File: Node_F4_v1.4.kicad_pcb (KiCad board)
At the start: 2 copper layers, 95 x 58.5 mm, 84 parts, among them J1 Screw_Terminal_01x09, J6 Conn_01x16_Female, J7 Conn_01x08_Male, J8 STLINK, Q1 P_Mosfet, SW1 SW_Push, U10 Ai-Thinker-Ra-02, U2 PCF8574A, U3 AMS1117-3.3, U4 DS3231M, U5 MAX485E, U6 STM32F411CEUx, U7 Trans_MOSFET, U8 Trans_MOSFET, U9 W25Q128JVS, Y1 25MHz

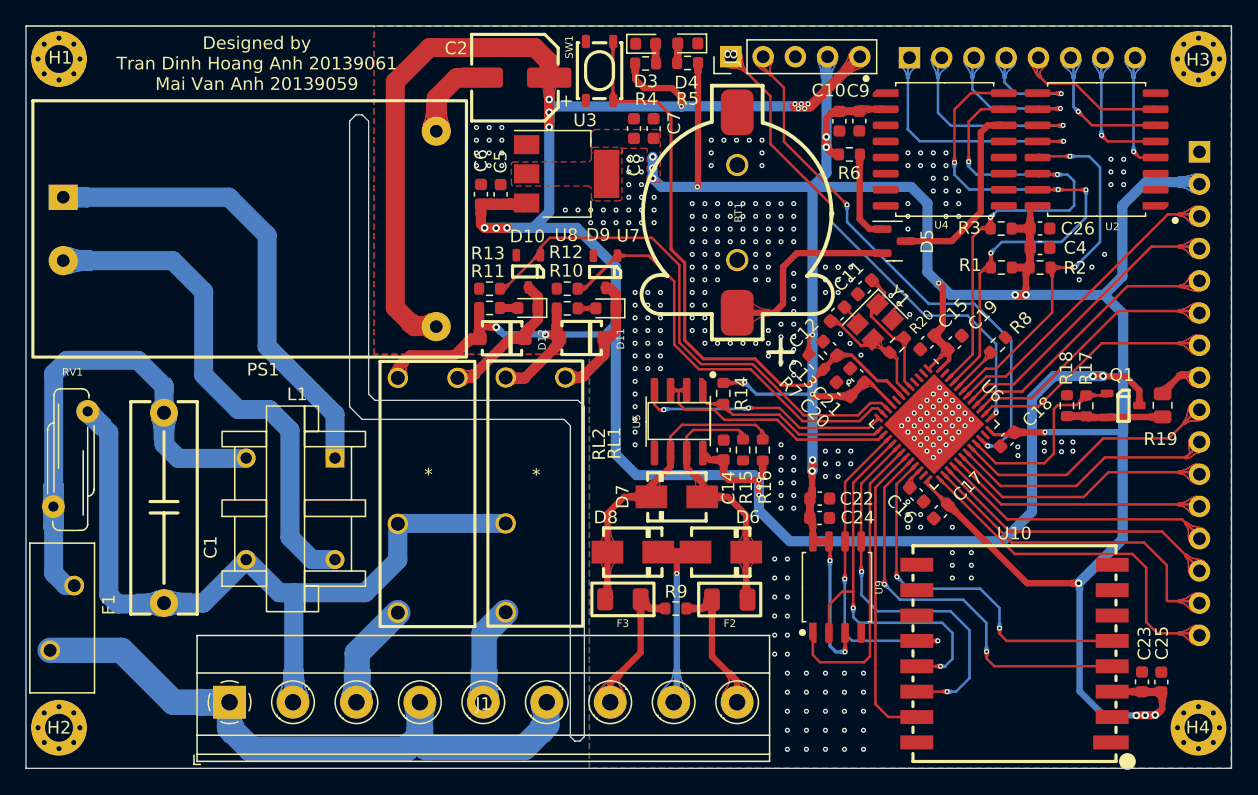
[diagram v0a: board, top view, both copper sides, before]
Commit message: chinh via
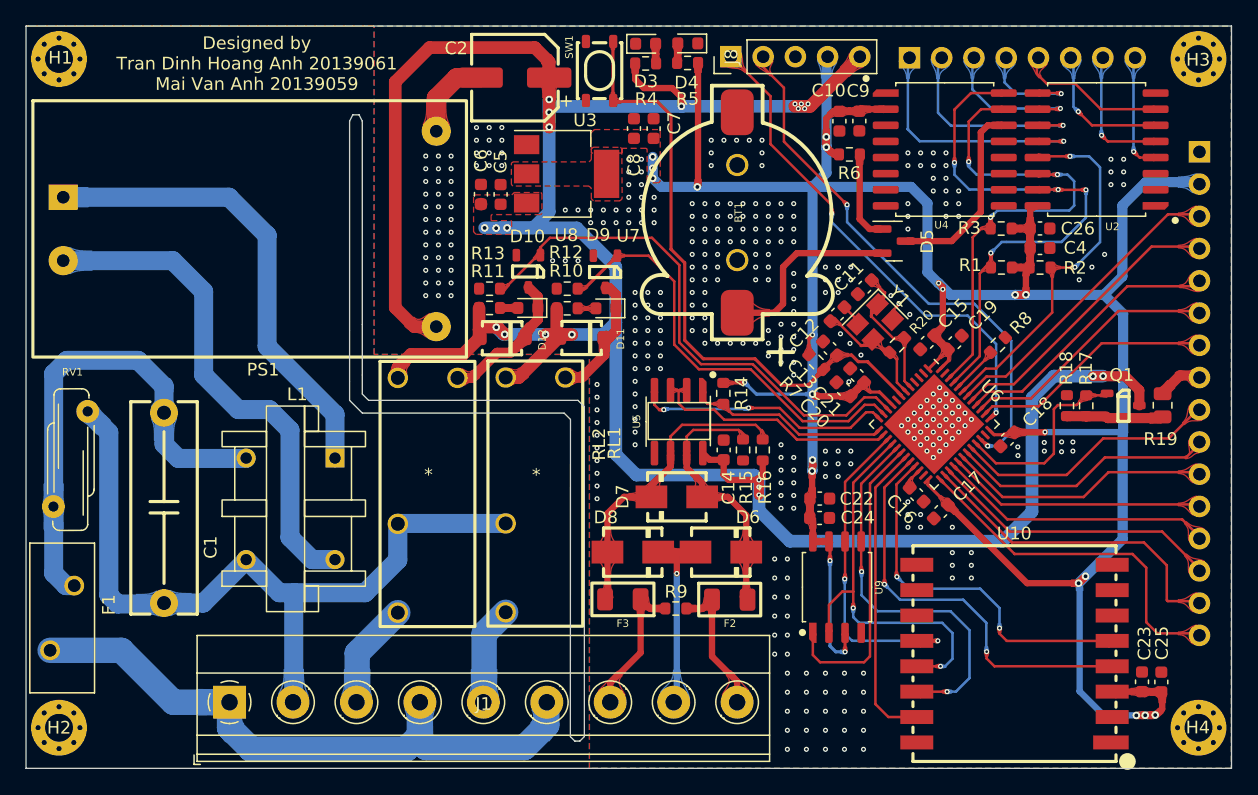
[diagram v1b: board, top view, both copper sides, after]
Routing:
- net +5V: track 222.5 -> 217.0 mm, vias 19 -> 21
- net +3.3V: track 241.8 -> 242.7 mm, vias 21 -> 23
- net GND: vias 314 -> 363
- added copper zone on F.Cu, net +5V
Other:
- outline, holes or cut-outs redrawn

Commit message: DONE
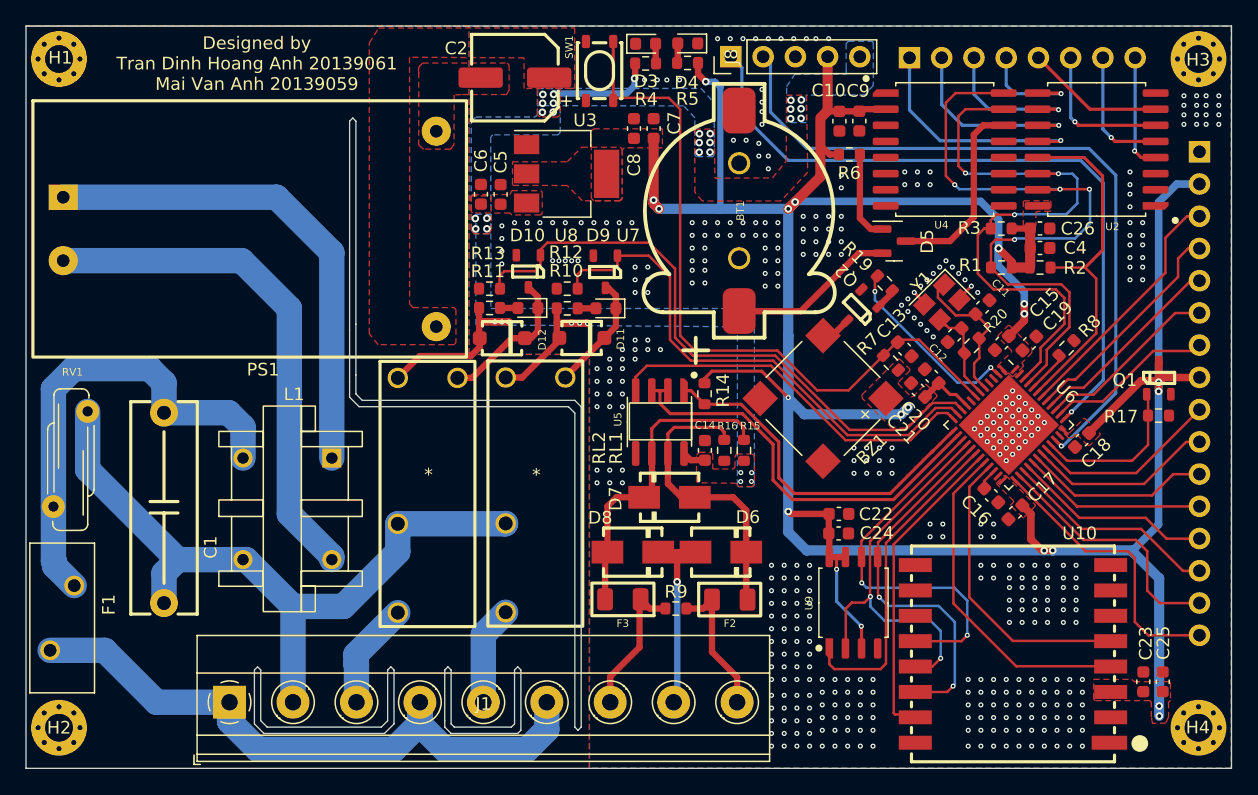
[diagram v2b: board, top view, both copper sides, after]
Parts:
- removed R18: 1K, Resistor_SMD:R_0603_1608Metric
- added BZ1: Buzzer, Buzzer_Beeper:PUIAudio_SMT_0825_S_4_R, F.Cu at (140.3, 78.8)
- added Q2: MMBT3904L, IVS_FOOTPRINTS:SOT23-3, F.Cu at (144.5, 71.8)
- R19: value 100R -> 1K; footprint Resistor_SMD:R_0805_2012Metric -> Resistor_SMD:R_0603_1608Metric
- moved R19 23.9 mm to (145.2, 69.8), turned to 135 degrees
- moved C11 9.41 mm to (152.9, 71.7), turned to -135 degrees
- moved C12 9.38 mm to (150.7, 73.9), turned to 45 degrees
- moved C21 5.88 mm to (147.8, 78.2)
- moved C13 5.88 mm to (146.7, 75.0), turned to 135 degrees
- moved C15 5.88 mm to (154.4, 74.5)
- moved C16 5.88 mm to (153.6, 86.5)
- moved C17 5.88 mm to (155.5, 87.8)
- moved C18 5.88 mm to (160.7, 82.1)
- moved C19 5.88 mm to (156.6, 74.5)
- moved C20 5.88 mm to (148.9, 77.1)
- moved R20 5.88 mm to (152.0, 74.7)
- moved R7 5.88 mm to (145.7, 76.0), turned to 135 degrees
- moved U6 5.88 mm to (154.9, 80.9)
- moved R17 5.75 mm to (166.8, 80.2), turned to 180 degrees
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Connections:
- J6 pad 8: Net-(J6-Pad8) -> +3.3V
- Q1 pad 2: Net-(Q1-Pad2) -> GND
- Q1 pad 3: +5V -> +3.3V
- R17 pad 1: Net-(Q1-Pad2) -> GND
- R19 pad 1: Net-(Q1-Pad2) -> Net-(Q2-Pad1)
- R19 pad 2: Net-(J6-Pad8) -> /BUZZER
- U6 pad 2: unconnected-(U6-Pad2) -> /BUZZER
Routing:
- net +5V: track 217.0 -> 33.5 mm, vias 21 -> 33
- net /SWCLK: track 39.4 -> 55.5 mm, vias 2 -> 1
- net /BUZZER: track 0.00 -> 15.1 mm, vias 0 -> 2
- net /SWDIO: track 42.8 -> 57.7 mm, vias 2 -> 1
- net /RS485_DERE: track 19.8 -> 32.6 mm
- net /RX_RS485: track 15.9 -> 28.5 mm
- net /TX_RS485: track 20.4 -> 30.0 mm, vias 2 -> 0
- net /SDA: track 40.4 -> 48.7 mm
- net /SCL: track 44.5 -> 52.7 mm
- net Net-(C13-Pad2): track 48.7 -> 56.8 mm
- net /RELAY_2: track 34.3 -> 42.0 mm
- net Net-(Q1-Pad2): track 7.52 -> 0.00 mm
- net /RELAY_1: track 42.9 -> 49.7 mm
- net Net-(C2-Pad2): track 6.78 -> 0.00 mm
- net /TFT_DB2: track 20.9 -> 14.7 mm
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- added copper zone on B.Cu, net +5V
- added copper zone on F.Cu, net Net-(C2-Pad2)
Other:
- outline, holes or cut-outs redrawn
- board text added: "5v 3v3 GND DIO SCK"
- board text added: "B- EARTH A+"
- board text removed: "5v 3v3 GND DIO CLK"
- board text removed: "B- GND A+"
